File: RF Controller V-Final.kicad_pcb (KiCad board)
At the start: 2 copper layers, 132 x 67.5 mm, 41 parts, among them J2 J_OLED, J3 BAT+, J4 BAT-, SW1 EG1218, U1 Teensy4.0, U3 NRF24L01, U5 AP2112K-3.3, U7 Pitch/Roll, U8 TPS542025DDCR, U9 Throttle/Yaw

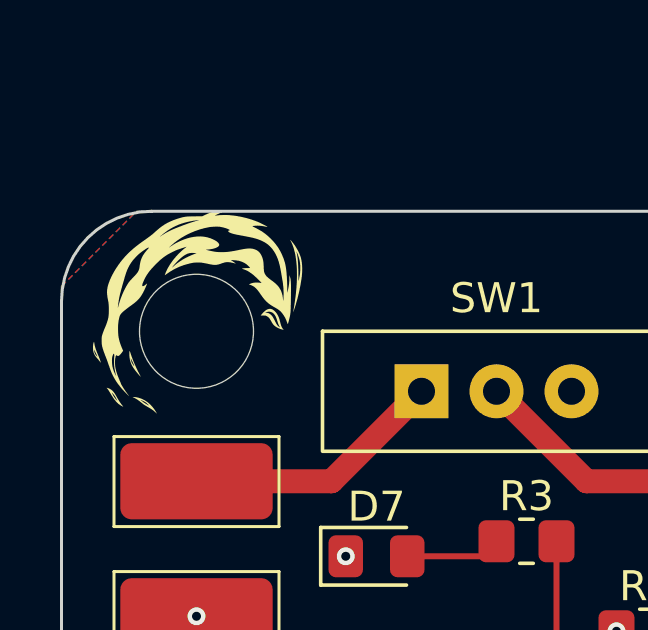
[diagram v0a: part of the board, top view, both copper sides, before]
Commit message: prev change was not saved
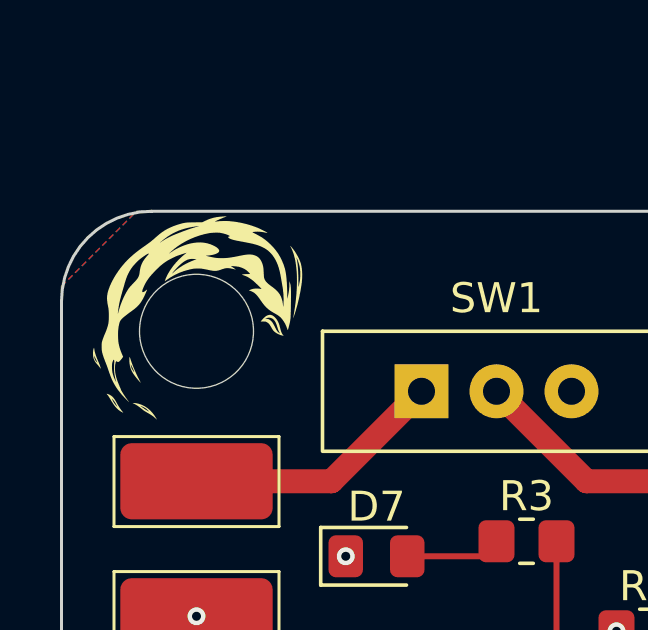
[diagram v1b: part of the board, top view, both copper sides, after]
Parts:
- moved ? 0.20 mm to (86.5, 71.5)
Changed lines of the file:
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@@
 	(footprint "RF_MountingHoles:holeborderart"
 		(layer "F.Cu")
-		(at 86.5 71.3)
+		(at 86.5 71.5)
 		(property "Reference" ""
 			(at 0 0 0)
